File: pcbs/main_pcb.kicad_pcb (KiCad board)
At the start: 2 copper layers, 139.3 x 147.8 mm, 60 parts

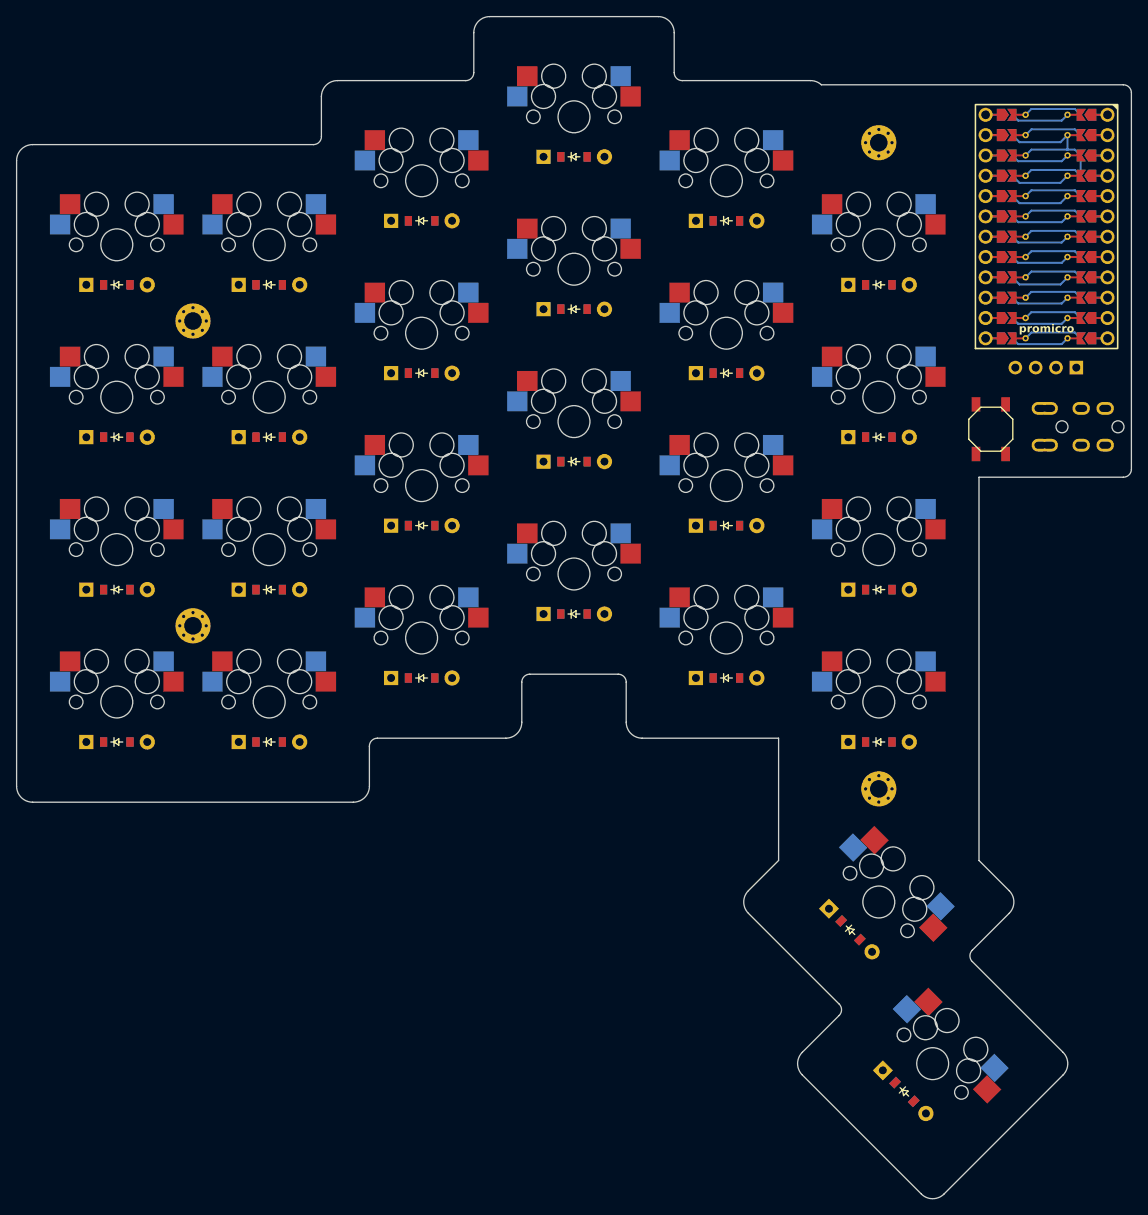
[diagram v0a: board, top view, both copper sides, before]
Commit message: gerbers
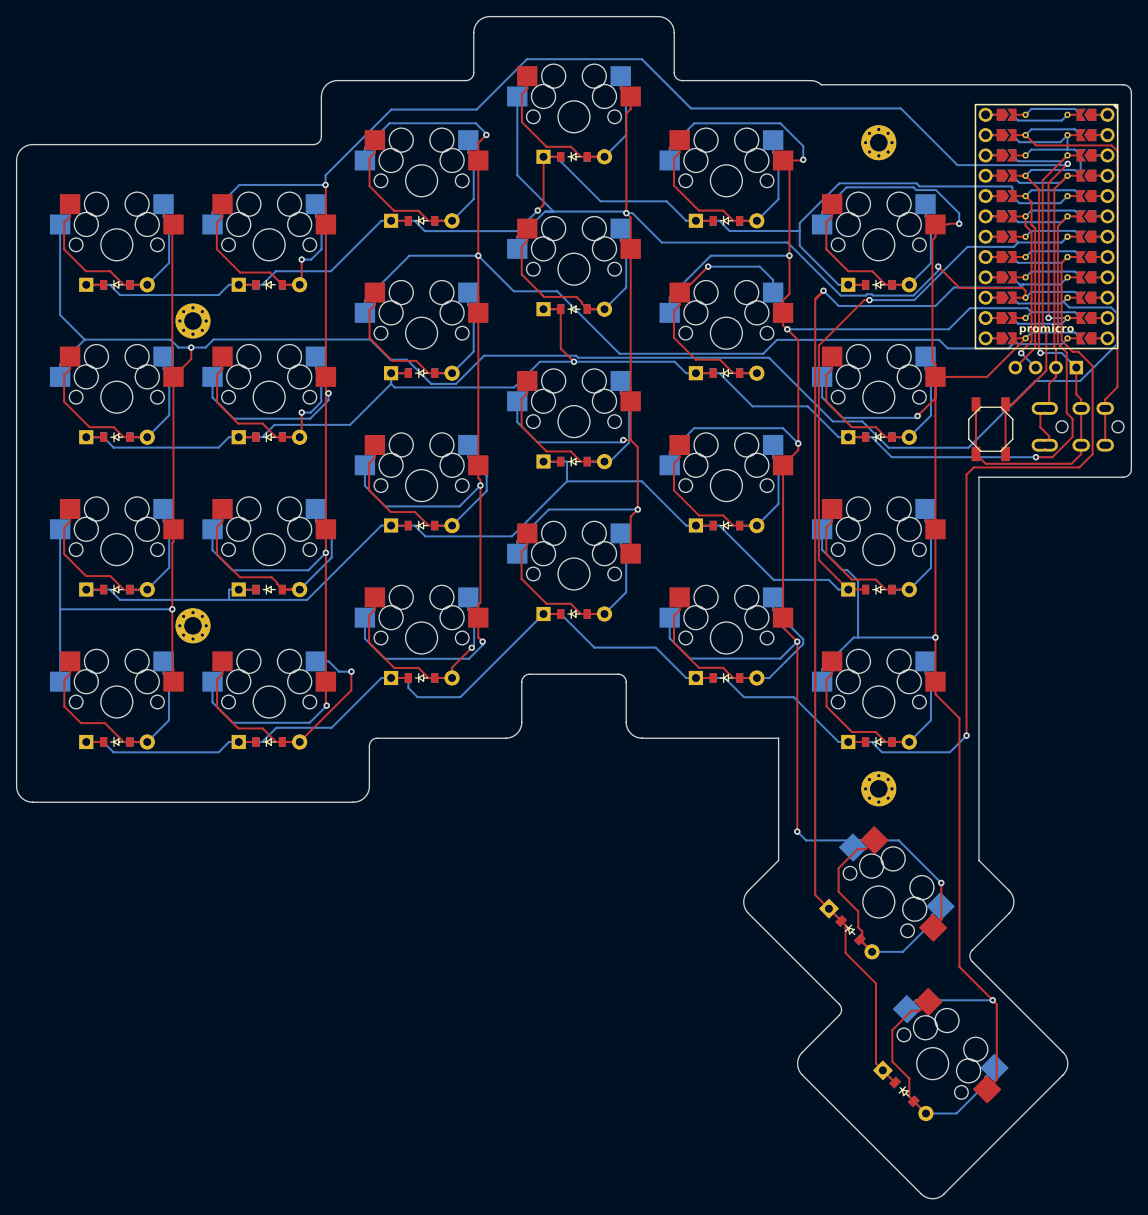
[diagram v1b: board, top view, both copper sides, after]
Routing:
- net P14: track 9.20 -> 280.8 mm, vias 0 -> 2
- net P16: track 9.20 -> 278.2 mm, vias 0 -> 6
- net P8: track 9.13 -> 241.4 mm, vias 0 -> 7
- net P18: track 9.13 -> 228.1 mm, vias 0 -> 1
- net P9: track 9.13 -> 226.6 mm, vias 0 -> 4
- net P10: track 9.13 -> 225.7 mm, vias 0 -> 4
- net P19: track 9.13 -> 203.1 mm, vias 0 -> 1
- net P20: track 9.13 -> 199.8 mm, vias 0 -> 2
- net P7: track 9.13 -> 195.5 mm, vias 0 -> 4
- net P21: track 9.26 -> 170.9 mm, vias 0 -> 1
- net P15: track 9.26 -> 149.9 mm, vias 0 -> 1
- net GND: track 31.9 -> 93.0 mm, vias 0 -> 1
- net P0: track 9.13 -> 58.8 mm
- net RST: track 9.13 -> 50.5 mm
- net VCC: track 9.26 -> 46.7 mm
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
